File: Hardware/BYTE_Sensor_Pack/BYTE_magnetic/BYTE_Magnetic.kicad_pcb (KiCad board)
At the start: 2 copper layers, 18 x 23 mm, 20 parts, among them J1 Input, M1 Motor_DC, U1 DRV2605LDGS, U2 ADS1115IDGS, U3 PTCA9536BDTMR, U4 SI7210-B-12-IM2, U5 SI7210-B-13-IM2, U6 SI7210-B-14-IM2

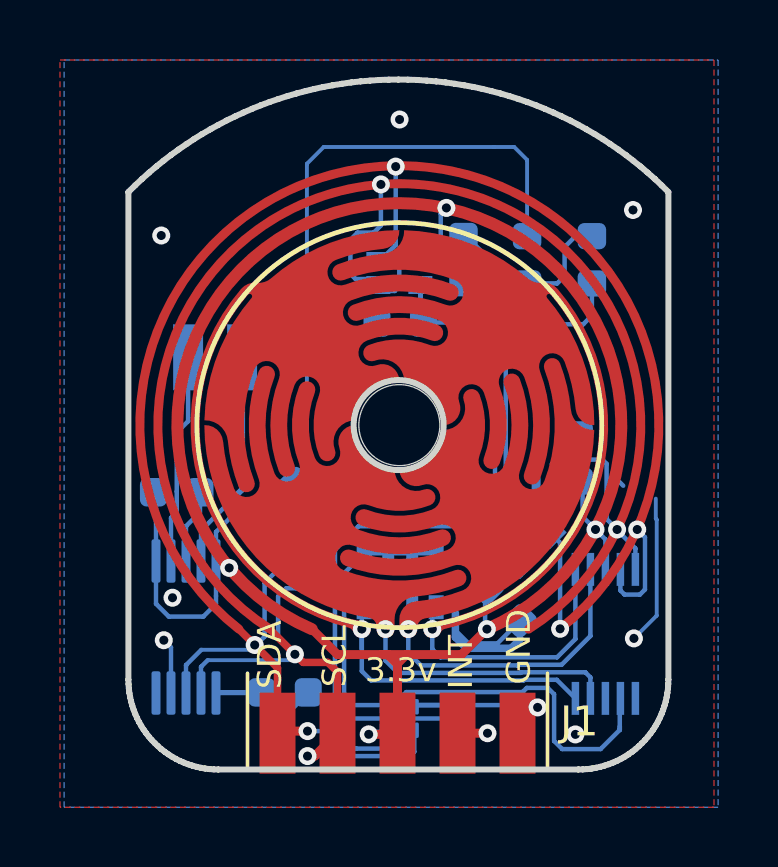
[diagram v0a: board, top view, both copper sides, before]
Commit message: update magnetic pcb and
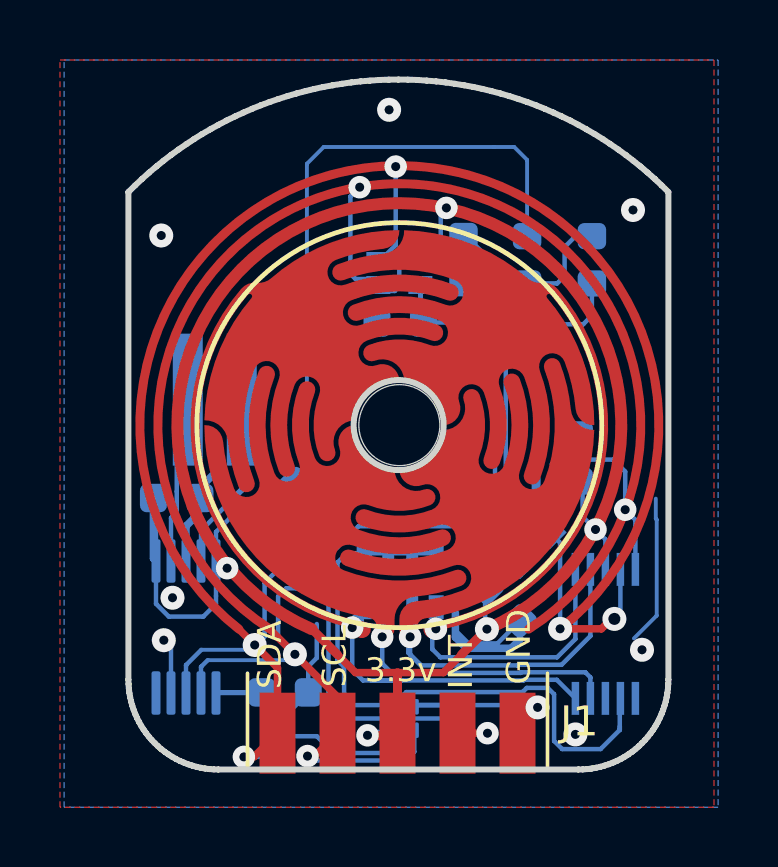
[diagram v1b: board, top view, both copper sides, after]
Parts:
- moved M1 1.51 mm to (176.9, 112.0)
- moved C5 0.19 mm to (174.6, 114.1)
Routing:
- net GND: track 32.9 -> 37.7 mm
- net +3V3: track 39.4 -> 42.3 mm
- net /SDA: track 25.4 -> 28.2 mm
- net /A3: track 10.9 -> 13.0 mm
- net /A0: track 9.60 -> 11.2 mm
- net /A1: track 10.3 -> 11.9 mm
- net Net-(M1-Pad2): track 7.36 -> 5.83 mm
- net /SCL: track 32.3 -> 31.5 mm
- net /FSR_CTRL: track 8.94 -> 9.46 mm
